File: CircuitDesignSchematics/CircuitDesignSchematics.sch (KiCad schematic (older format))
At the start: 8 parts, among them P1 Power, P2 Analog, P3 Digital, P4 Digital, P5 CONN_01X01, P6 CONN_01X01, P7 CONN_01X01, P8 CONN_01X01

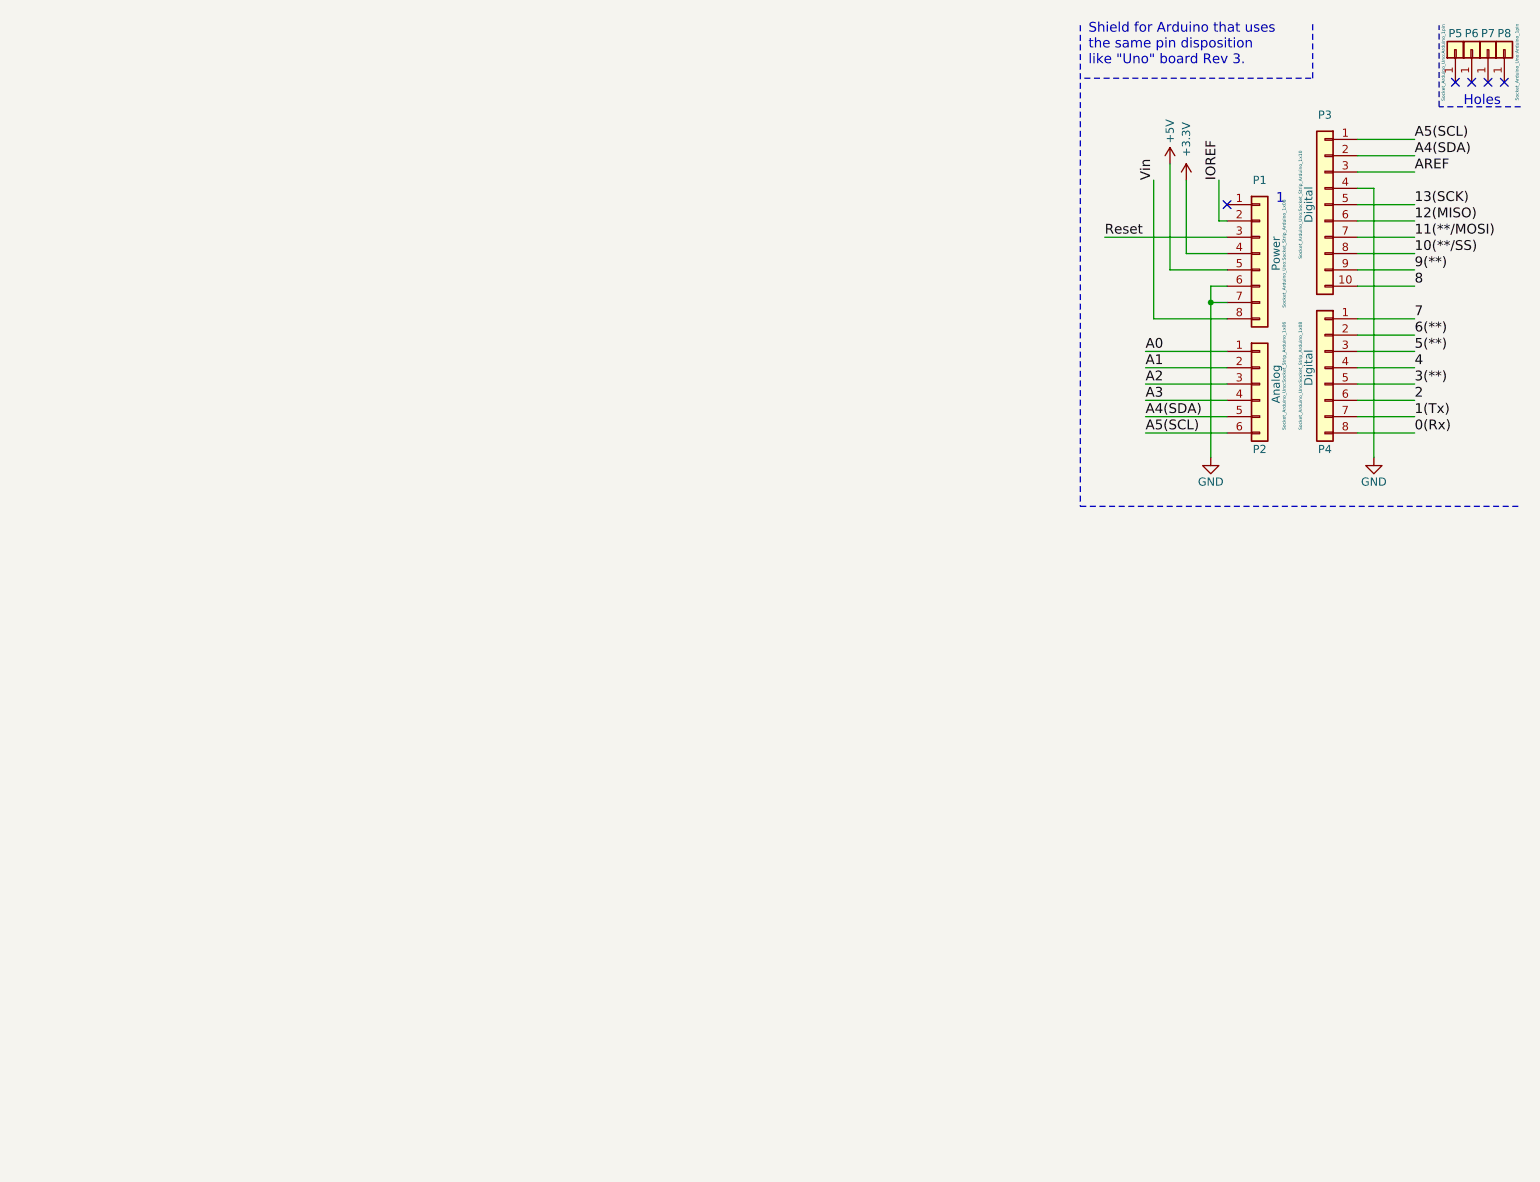
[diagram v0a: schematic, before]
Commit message: update schematics design
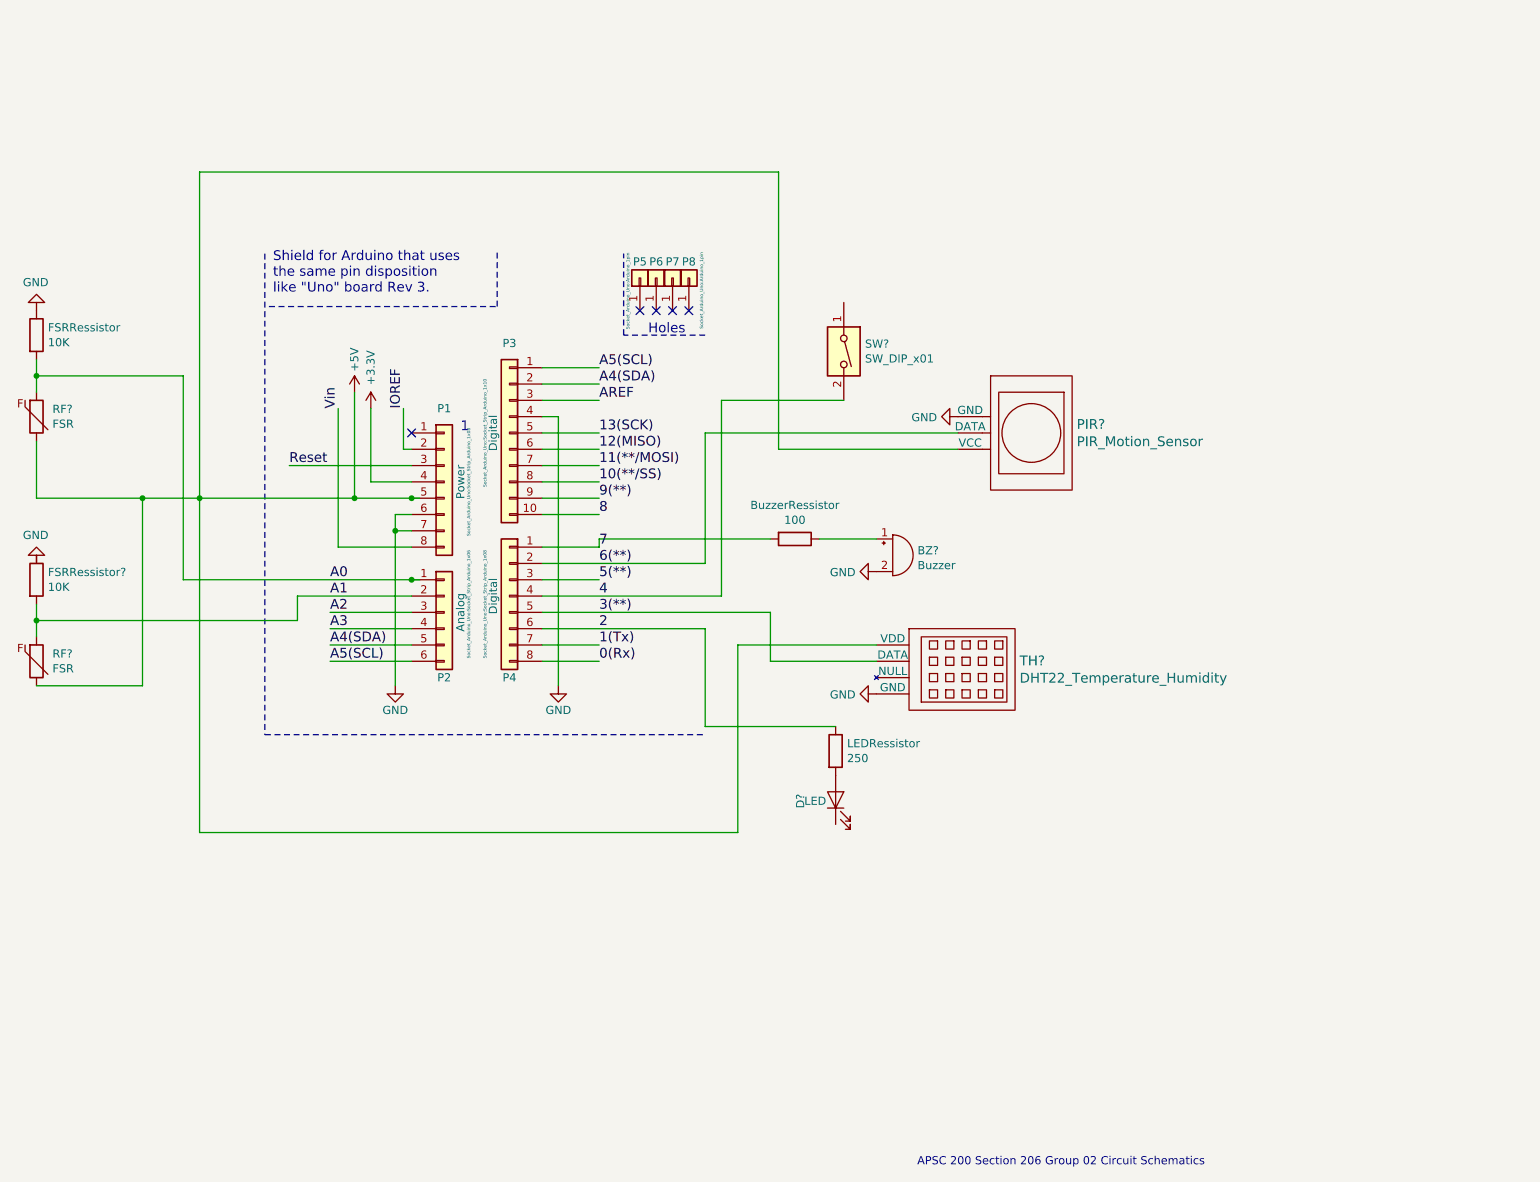
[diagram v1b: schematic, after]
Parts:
- added BZ?: Buzzer, symbol Device:Buzzer
- added BuzzerRessistor: 100, symbol Device:R
- added D?: LED, symbol Device:LED
- added FSRRessistor, FSRRessistor?: 10K, symbol Device:R
- added LEDRessistor: 250, symbol Device:R
- added PIR?: PIR_Motion_Sensor, symbol sensors:PIR_Motion_Sensor
- added RF? (x2): FSR, symbol fsr:FSR
- added SW?: SW_DIP_x01, symbol Switch:SW_DIP_x01
- added TH?: DHT22_Temperature_Humidity, symbol sensors:DHT22_Temperature_Humidity
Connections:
- net +5V: now also PIR?.3 (VCC), RF?.2, RF?.2, TH?.1 (VDD)
- net 2: now also LEDRessistor.1
- net 3(**): now also TH?.2 (DATA)
- net 4: now also SW?.2
- net 6(**): now also PIR?.2 (DATA)
- net 7: now also BuzzerRessistor.2
- net A0: now also FSRRessistor.2, RF?.1
- net A1: now also FSRRessistor?.2, RF?.1
- net GND: now also BZ?.2 (+), FSRRessistor.1, PIR?.1 (GND), TH?.4 (GND)
- new net: BZ?.1 (-), BuzzerRessistor.1
- new net: D?.2 (A), LEDRessistor.2
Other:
- note added: "APSC 200 Section 206 Group 02 Circuit Schematics"
- moved on the sheet: P1, P2, P3, P4, P5, P6, P7, P8
